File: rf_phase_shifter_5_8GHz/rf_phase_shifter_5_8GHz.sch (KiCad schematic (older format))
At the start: 12 parts, among them J1 Conn_Coaxial, J2 Conn_Coaxial, J3 Conn_Coaxial

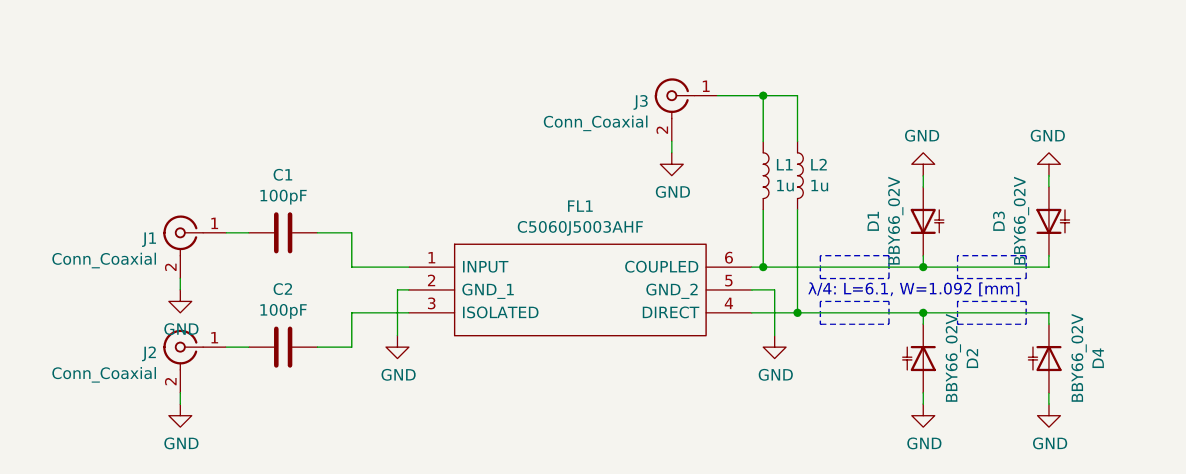
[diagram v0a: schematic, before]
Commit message: updated libs
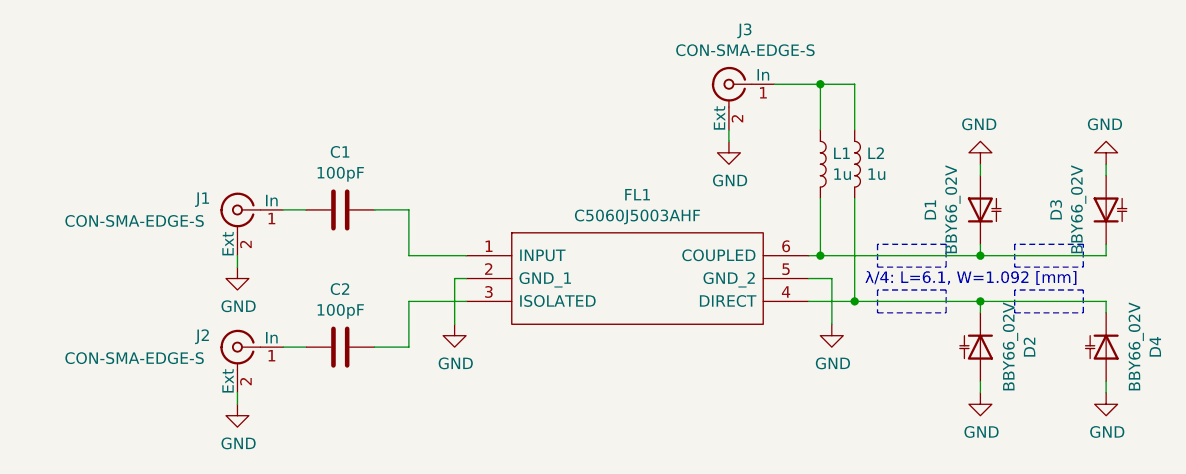
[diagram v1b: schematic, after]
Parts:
- removed J1, J2, J3: Conn_Coaxial, Connector_Coaxial:SMA_Samtec_SMA-J-P-X-ST-EM1_EdgeMount, symbol Connector:Conn_Coaxial
- added J1, J2, J3: CON-SMA-EDGE-S, analog_rf_phase_shifter_module:CON-SMA-EDGE-S, symbol analog_rf_phase_shifter_module:CON-SMA-EDGE-S
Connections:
- net GND: now also J1.2 (Ext), J2.2 (Ext), J3.2 (Ext)
- net at L1.1, L2.1: now also J3.1 (In)
- net at C2.1: now also J2.1 (In)
- net at C1.2: now also J1.1 (In)
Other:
- moved on the sheet: C1, C2, D1, D2, D3, D4, FL1, L1, L2
